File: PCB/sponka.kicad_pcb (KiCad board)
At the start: 2 copper layers, 59.3 x 10.9 mm, 30 parts, among them J1 Conn_01x03_Pin, J2 USB_C_Receptacle_USB2.0_14P, J3 Conn_01x02_Socket, J4 Conn_01x05_Pin, SW1 SW_Push, SW2 SW_SPDT, U1 CH32V003FxUx, U2 TP4057, U3 AP2127K-3.3

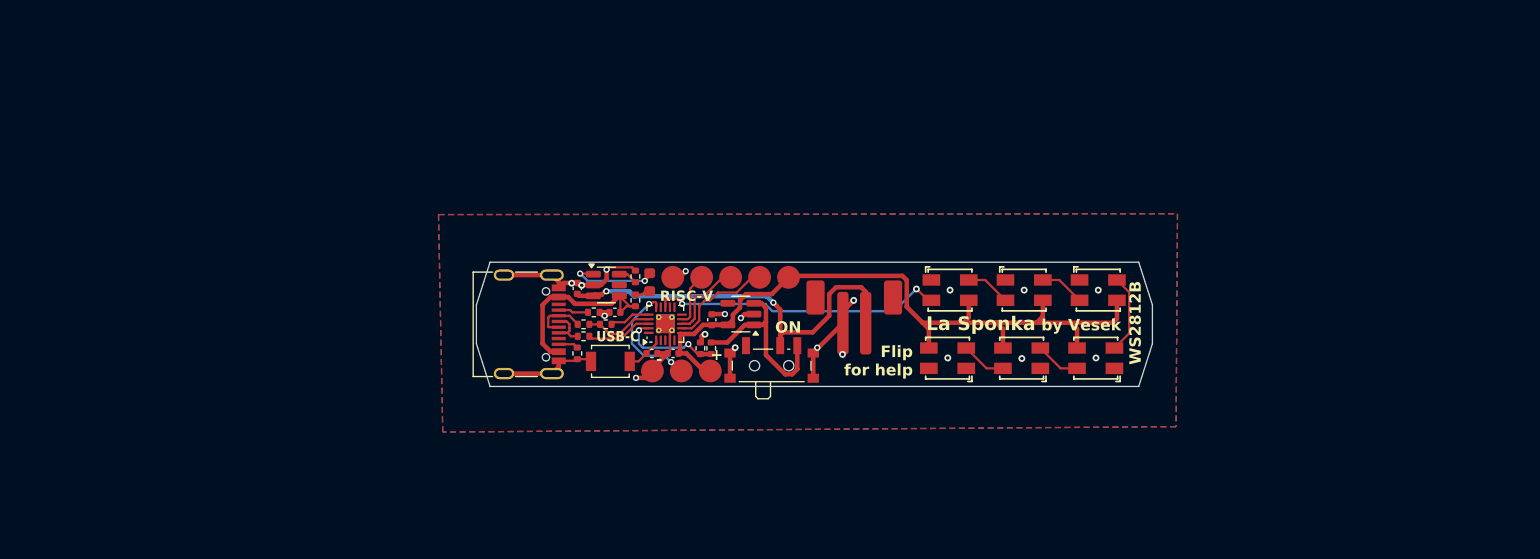
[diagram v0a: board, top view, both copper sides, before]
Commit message: New design WIP
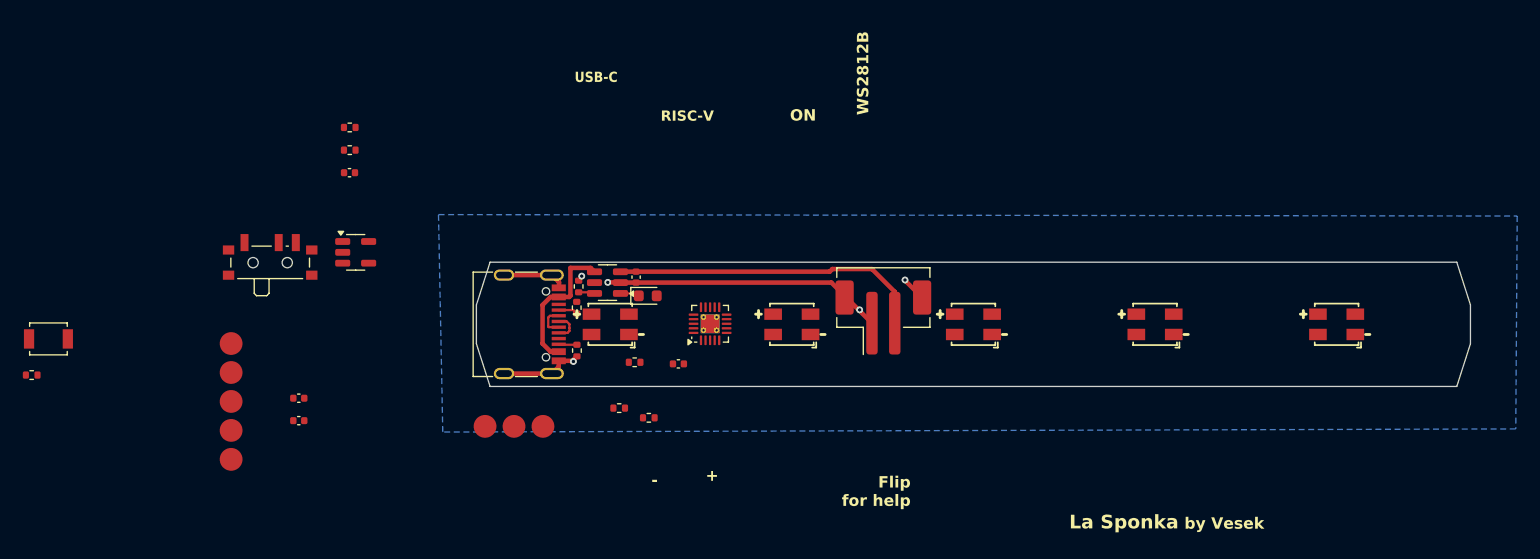
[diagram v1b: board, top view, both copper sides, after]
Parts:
- removed LED6: WS2812B-MINI, sponka:LED-SMD_4P-L3.5-W3.5-TL_WS2812B
- moved R9 50.6 mm to (61.7, 105.8), turned to 0 degrees
- moved SW1 49.3 mm to (63.2, 102.6), turned to 0 degrees
- moved J4 45.2 mm to (79.2, 108.1), turned to 0 degrees
- moved SW2 44.9 mm to (82.6, 95.6)
- moved R7 37.2 mm to (89.6, 84.1), turned to 0 degrees
- moved R8 35.3 mm to (89.6, 86.1), turned to 0 degrees
- moved C5 34.3 mm to (89.6, 88.0), turned to 0 degrees
- moved U3 34.2 mm to (90.1, 95.0), turned to 0 degrees
- moved C1 33.1 mm to (85.1, 107.8), turned to 0 degrees
- moved C2 31.5 mm to (85.1, 109.8), turned to 0 degrees
- moved LED1 30.0 mm to (112.4, 101.3), turned to 0 degrees
- moved LED5 27.8 mm to (176.2, 101.3)
- moved LED2 20.6 mm to (128.4, 101.3), turned to 0 degrees
- moved J1 15.5 mm to (104.0, 110.3), turned to -90 degrees
- moved LED3 11.4 mm to (144.3, 101.3), turned to 0 degrees
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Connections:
- J3 pad MP: (no net) -> GND
- LED5 pad 2: Net-(LED5-DOUT) -> unconnected-(LED5-DOUT-Pad2)
- SW2 pad : GND -> (no net)
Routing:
- net +3V3: track 64.2 -> 0.00 mm
- net /LED Row/Row_DIN: track 25.7 -> 0.00 mm, vias 2 -> 0
- net Net-(SW2-C): track 16.6 -> 0.00 mm
- net Net-(J1-Pin_2): track 11.2 -> 0.00 mm, vias 2 -> 0
- net /TX: track 9.42 -> 0.00 mm
- net /Power management/BATT_DIV: track 9.13 -> 0.00 mm, vias 2 -> 0
- net GND: track 48.0 -> 40.6 mm, vias 19 -> 5
- net Net-(J3-Pin_2): track 35.1 -> 27.7 mm, vias 2 -> 0
- net /RX/SDA: track 7.13 -> 0.00 mm
- net Net-(LED3-DOUT): track 6.95 -> 0.00 mm
- net Net-(D_CHRG1-K): track 8.02 -> 1.69 mm, vias 2 -> 0
- net /Power management/USB_DN: track 6.11 -> 0.00 mm
- net /Power management/USB_DP: track 5.84 -> 0.00 mm
- net /Power management/VBUS: track 17.5 -> 12.6 mm
- net /RTS/SCL: track 4.71 -> 0.00 mm
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- removed copper zone on F.Cu, net GND
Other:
- board size 59.3 x 10.9 mm -> 87.2 x 10.9 mm
